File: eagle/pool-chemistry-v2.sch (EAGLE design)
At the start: 17 parts, among them U1 ESP-WROOM-32

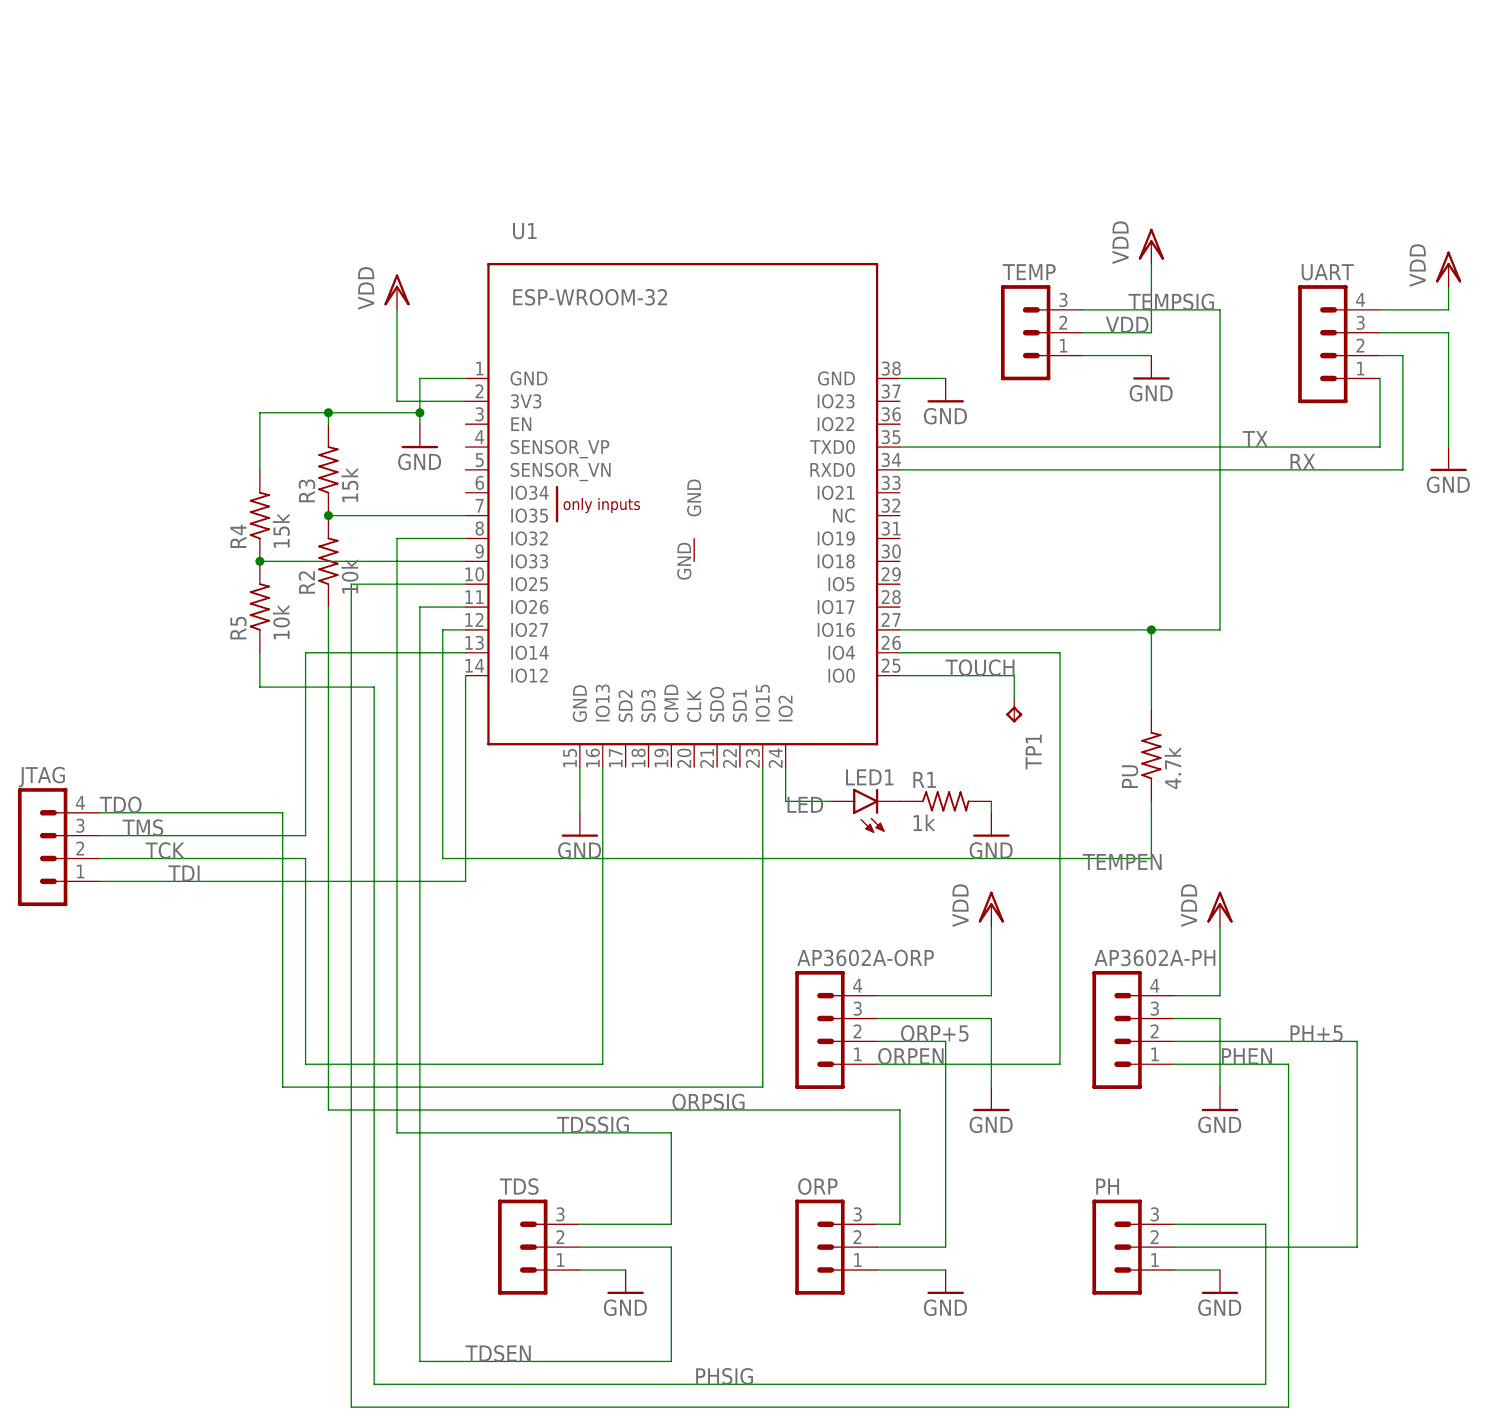
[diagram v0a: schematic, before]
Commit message: discrete components placed and routed
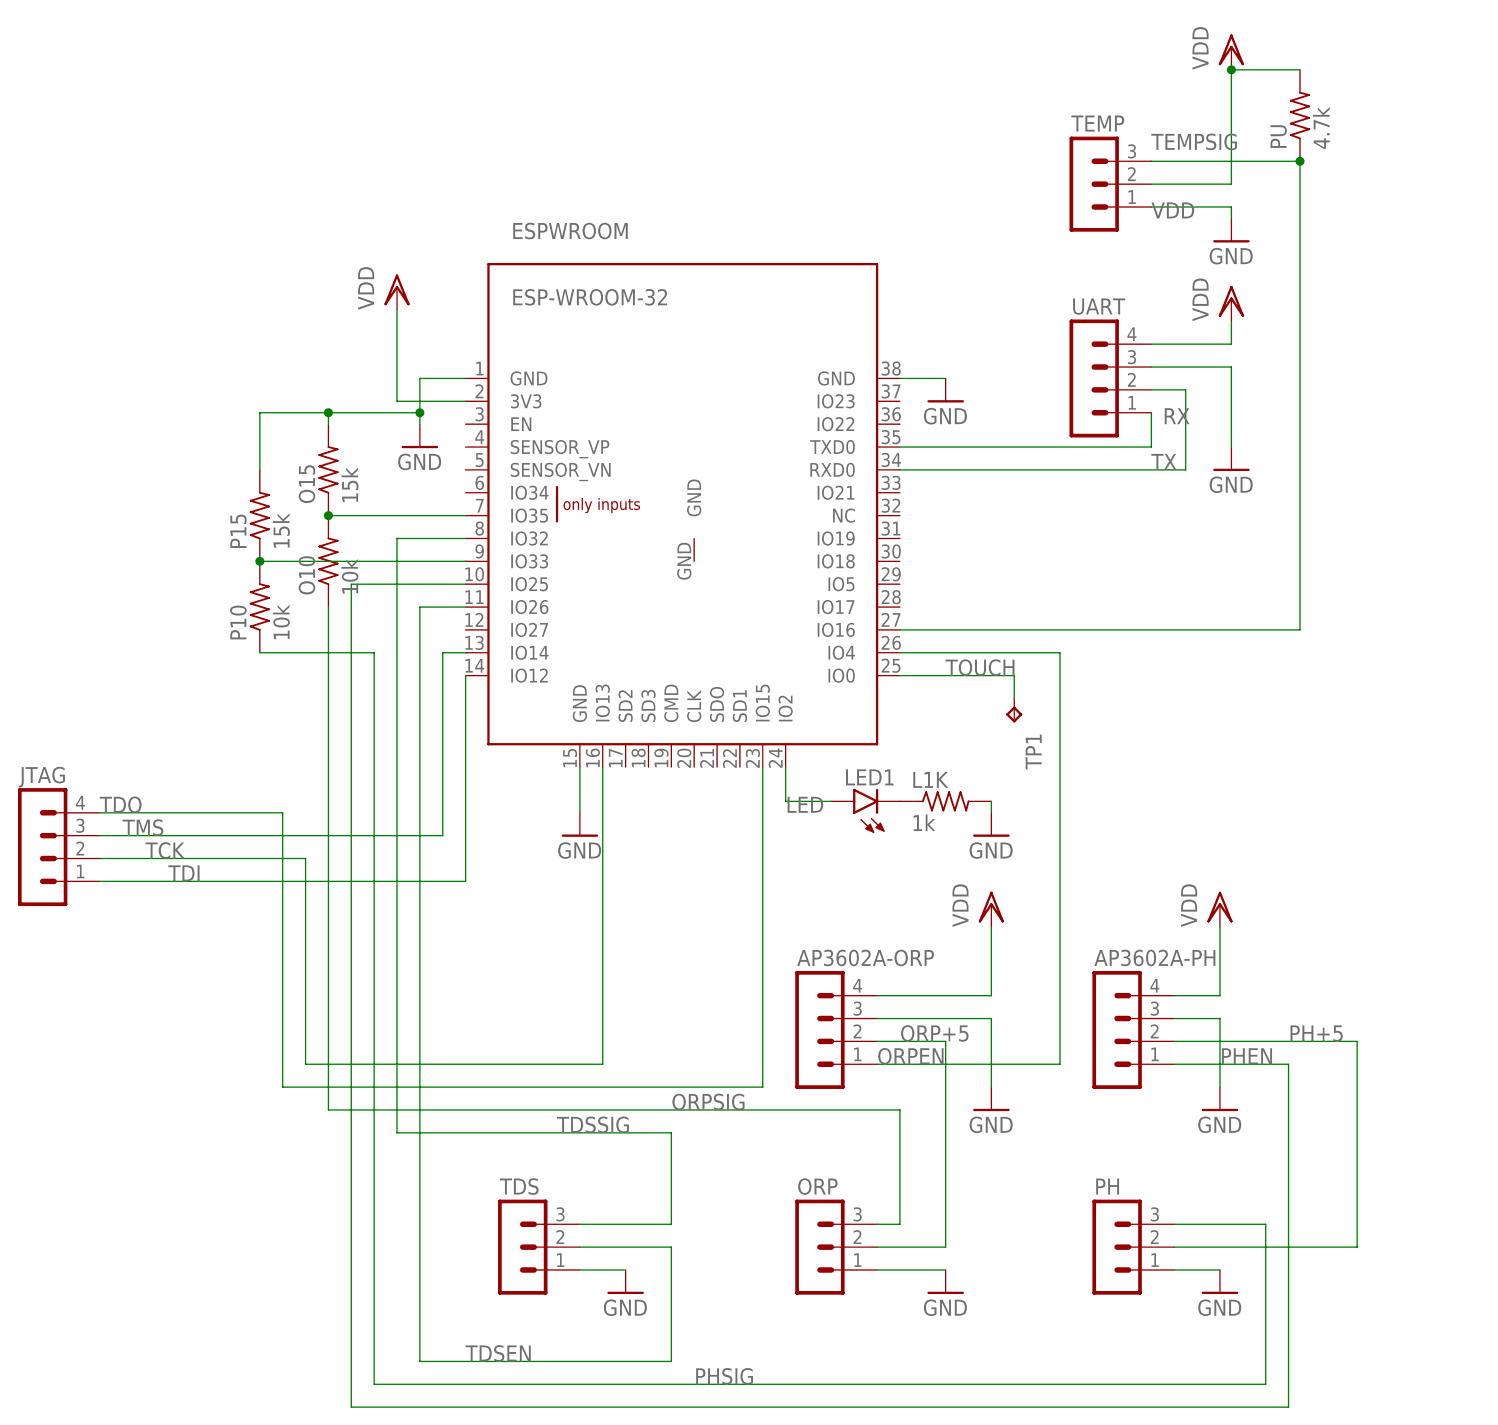
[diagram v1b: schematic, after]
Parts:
- renumbered R1 to L1K, R2 to O10, R3 to O15, R4 to P15, R5 to P10, U1 to ESPWROOM
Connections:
- removed net TEMPEN: ESPWROOM.IO27, PU.1
- net TEMPSIG: now also PU.1; no longer PU.2
- net VDD: now also PU.2
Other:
- moved on the sheet: PU, TEMP, UART
